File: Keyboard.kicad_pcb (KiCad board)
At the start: 2 copper layers, 50.8 x 59.5 mm, 37 parts, among them SW1 SW_Push, SW2 SW_Push, SW3 SW_Push, U1 ATmega32U2-AU, Y1 Crystal_GND24_Small

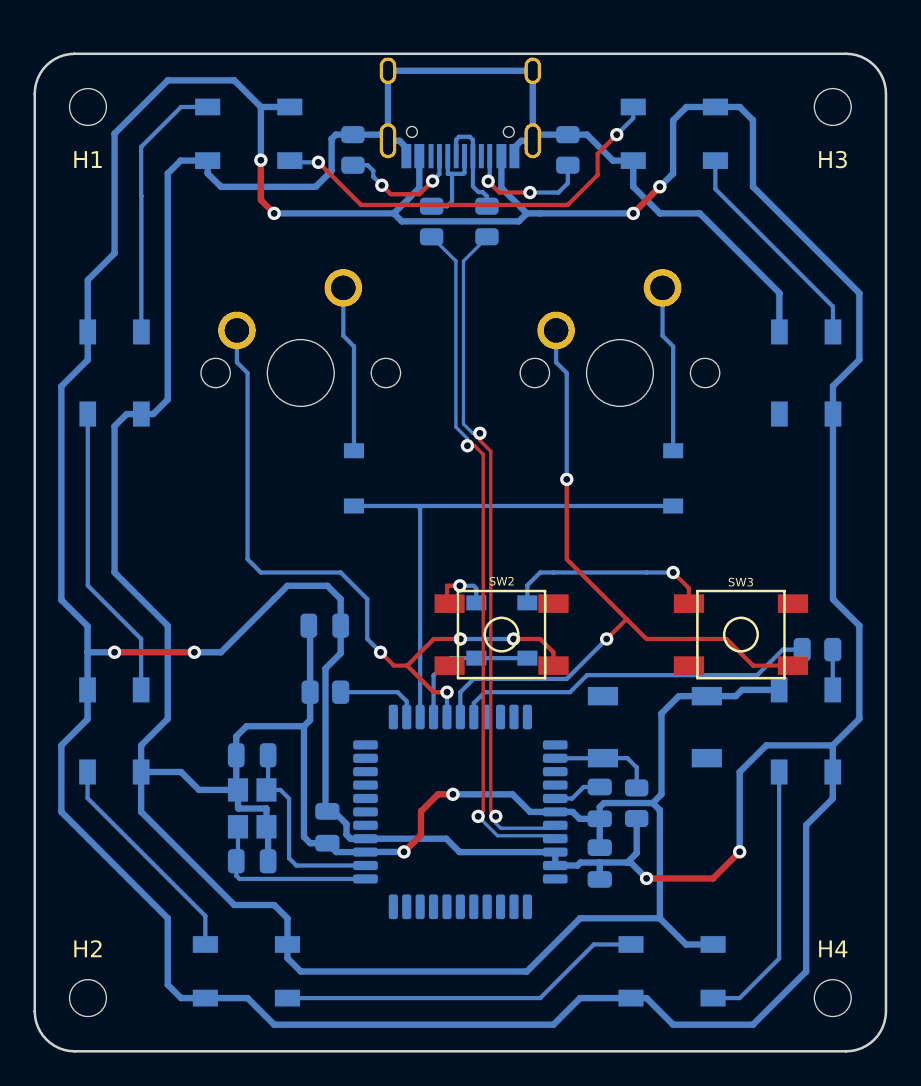
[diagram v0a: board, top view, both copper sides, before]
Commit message: sdfsdsdssdsdsssssdsds
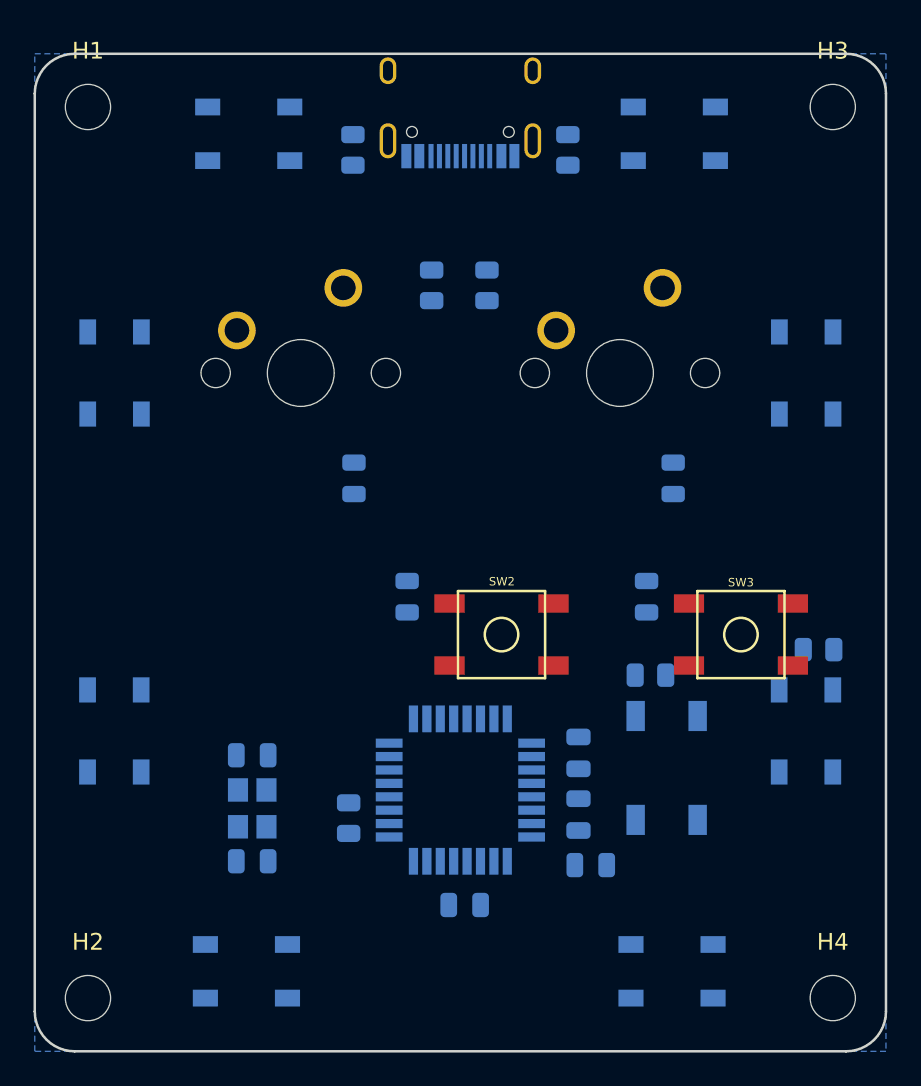
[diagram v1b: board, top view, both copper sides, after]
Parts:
- D1, D2, D3, D4: footprint Diode_SMD:D_SOD-123 -> Diode_SMD:D_0805_2012Metric
- H1, H2, H3, H4: footprint MountingHole:MountingHole_2.2mm_M2_DIN965 -> MountingHole:MountingHole_2.7mm_M2.5_DIN965
- U1: footprint Package_QFP:LQFP-44_10x10mm_P0.8mm -> Package_QFP:TQFP-32_7x7mm_P0.8mm
- moved C4 21.4 mm to (98.3, 86.5), turned to 0 degrees
- moved C5 9.42 mm to (90.7, 88.9), turned to 0 degrees
- moved R1 7.69 mm to (101.8, 75.2), turned to 0 degrees
- moved R4 7.64 mm to (83.8, 83.7), turned to 270 degrees
- moved D4 7.39 mm to (101.6, 70.5)
- moved D2 4.59 mm to (87.3, 70.5)
- moved R6 3.81 mm to (92.1, 51.9)
- moved R5 3.81 mm to (88.8, 51.9)
- moved C1 3.24 mm to (97.5, 79.8), turned to 270 degrees
- moved C6 3.19 mm to (97.5, 83.5)
- moved SW1 2.53 mm to (102.8, 80.7), turned to 90 degrees
- moved U1 1.30 mm to (90.5, 82.0), turned to 90 degrees
- moved R7 0.06 mm to (111.9, 73.7)
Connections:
- D11 pad 4: Net-(D10-Pad2) -> Net-(D11-Pad4)
- D5 pad 4: Net-(D5-Pad4) -> Net-(D12-Pad2)
- R7 pad 2: Net-(D5-Pad4) -> Net-(D11-Pad4)
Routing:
- net +5V: track 287.7 -> 0.00 mm, vias 8 -> 0
- net GND: track 223.3 -> 0.00 mm, vias 2 -> 0
- net COL1: track 43.3 -> 0.00 mm, vias 2 -> 0
- net COL0: track 42.5 -> 0.00 mm, vias 4 -> 0
- net D-: track 41.4 -> 0.00 mm, vias 2 -> 0
- net D+: track 40.3 -> 0.00 mm, vias 2 -> 0
- net ROW0: track 31.7 -> 0.00 mm
- net Net-(D10-Pad2): track 25.1 -> 0.00 mm, vias 2 -> 0
- net Net-(D6-Pad2): track 21.8 -> 0.00 mm
- net RGB: track 21.7 -> 0.00 mm
- net Net-(D8-Pad2): track 17.8 -> 0.00 mm
- net Net-(D5-Pad2): track 16.1 -> 0.00 mm
- net Net-(D10-Pad4): track 16.0 -> 0.00 mm
- net Net-(D7-Pad2): track 13.2 -> 0.00 mm
- net Net-(D11-Pad2): track 13.1 -> 0.00 mm
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- added copper zone on B.Cu, net GND
